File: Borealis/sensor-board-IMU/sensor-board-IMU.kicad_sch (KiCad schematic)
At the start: 6 parts, among them J2 Conn_01x03_Pin (data connecti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, J5 Conn_01x03_Pin (power connect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

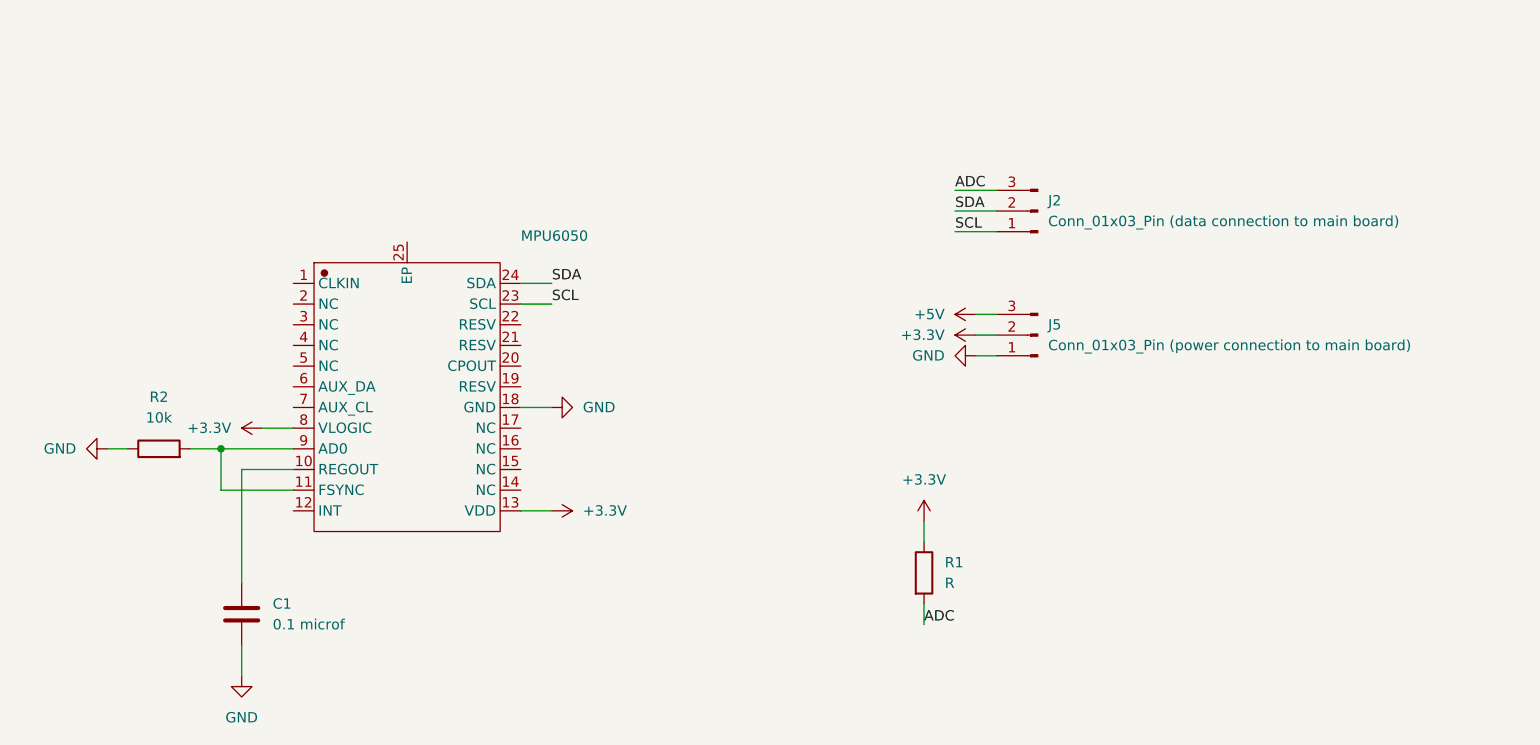
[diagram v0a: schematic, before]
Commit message: Fixed a few things
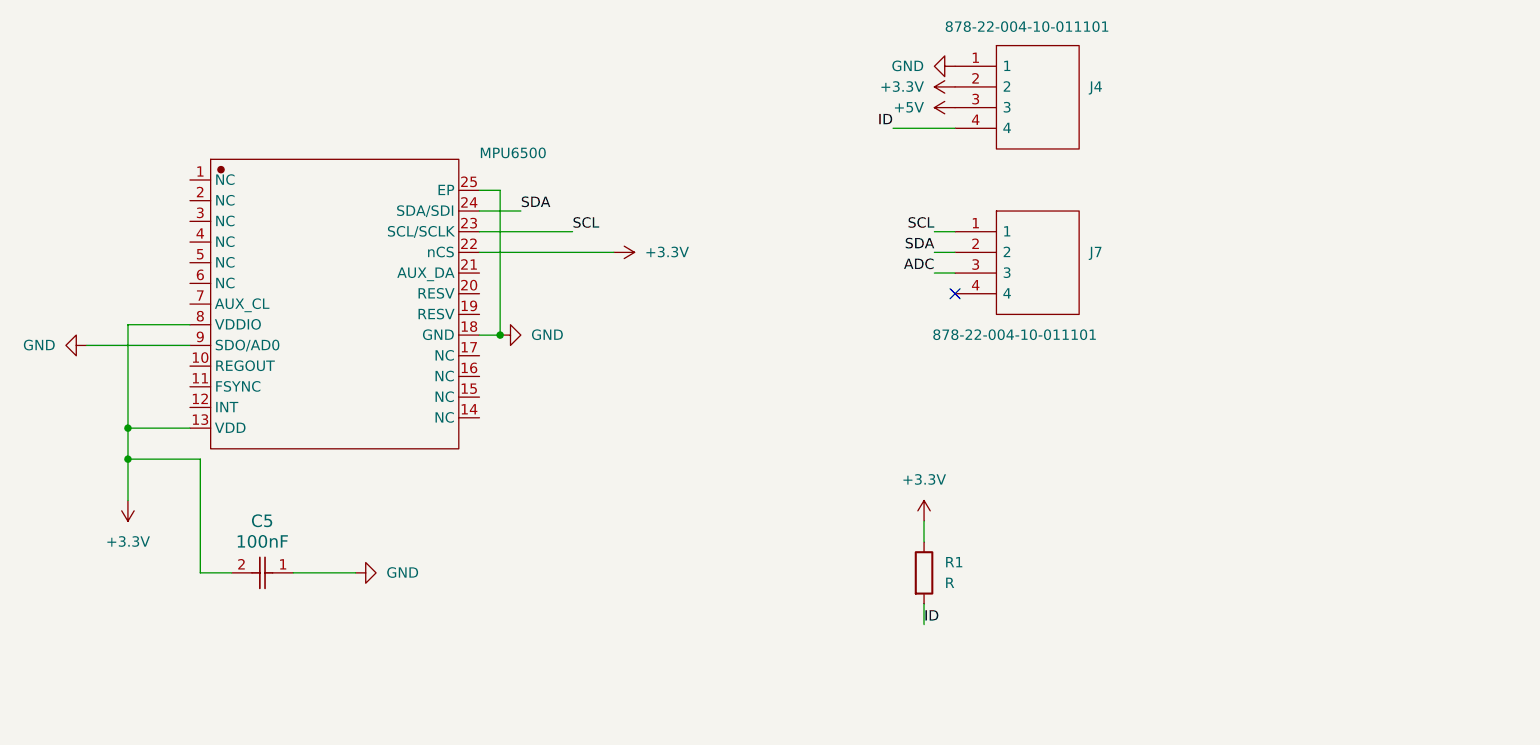
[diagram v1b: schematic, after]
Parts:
- removed C1: 0.1 microf, Capacitor_SMD:CP_Elec_3x5.3, symbol Device:C
- removed J2: Conn_01x03_Pin (data connection to main board), batteryholder:1x03 2.3 pitch, symbol Connector:Conn_01x03_Pin
- removed J5: Conn_01x03_Pin (power connection to main board), batteryholder:1x03 2.3 pitch, symbol Connector:Conn_01x03_Pin
- removed MPU6050: ~, batteryholder:MPU6050-footprint, symbol MPU-6050_C24112_2025-12-25-altium-import:root_0_MPU-6050_C24112_
- removed R2: 10k, Resistor_SMD:R_0805_2012Metric, symbol Device:R
- added C5: 100nF, BOREALIS:CAPC17595_95N_KEM, symbol 2026-01-23_05-30-51:C0603C104K5RACTU
- added J4, J7: 878-22-004-10-011101, BOREALIS:8782200410011101, symbol 878-22-004-10-011101:878-22-004-10-011101
- added MPU6500: ~, symbol mm-altium-import:root_0_MPU6500_
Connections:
- net +3.3V: now also C5.2, J4.2, MPU6500.13 (VDD), MPU6500.22 (nCS), MPU6500.8 (VDDIO)
- net +5V: now also J4.3
- net ADC: now also J7.3; no longer R1.2
- net GND: now also C5.1, J4.1, MPU6500.18 (GND), MPU6500.25 (EP), MPU6500.9 (SDO/AD0)
- net SCL: now also J7.1, MPU6500.23 (SCL/SCLK)
- net SDA: now also J7.2, MPU6500.24 (SDA/SDI)
- new net ID: J4.4, R1.2
- no-connect marks 0 -> 1
